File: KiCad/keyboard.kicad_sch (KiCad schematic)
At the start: 1 part

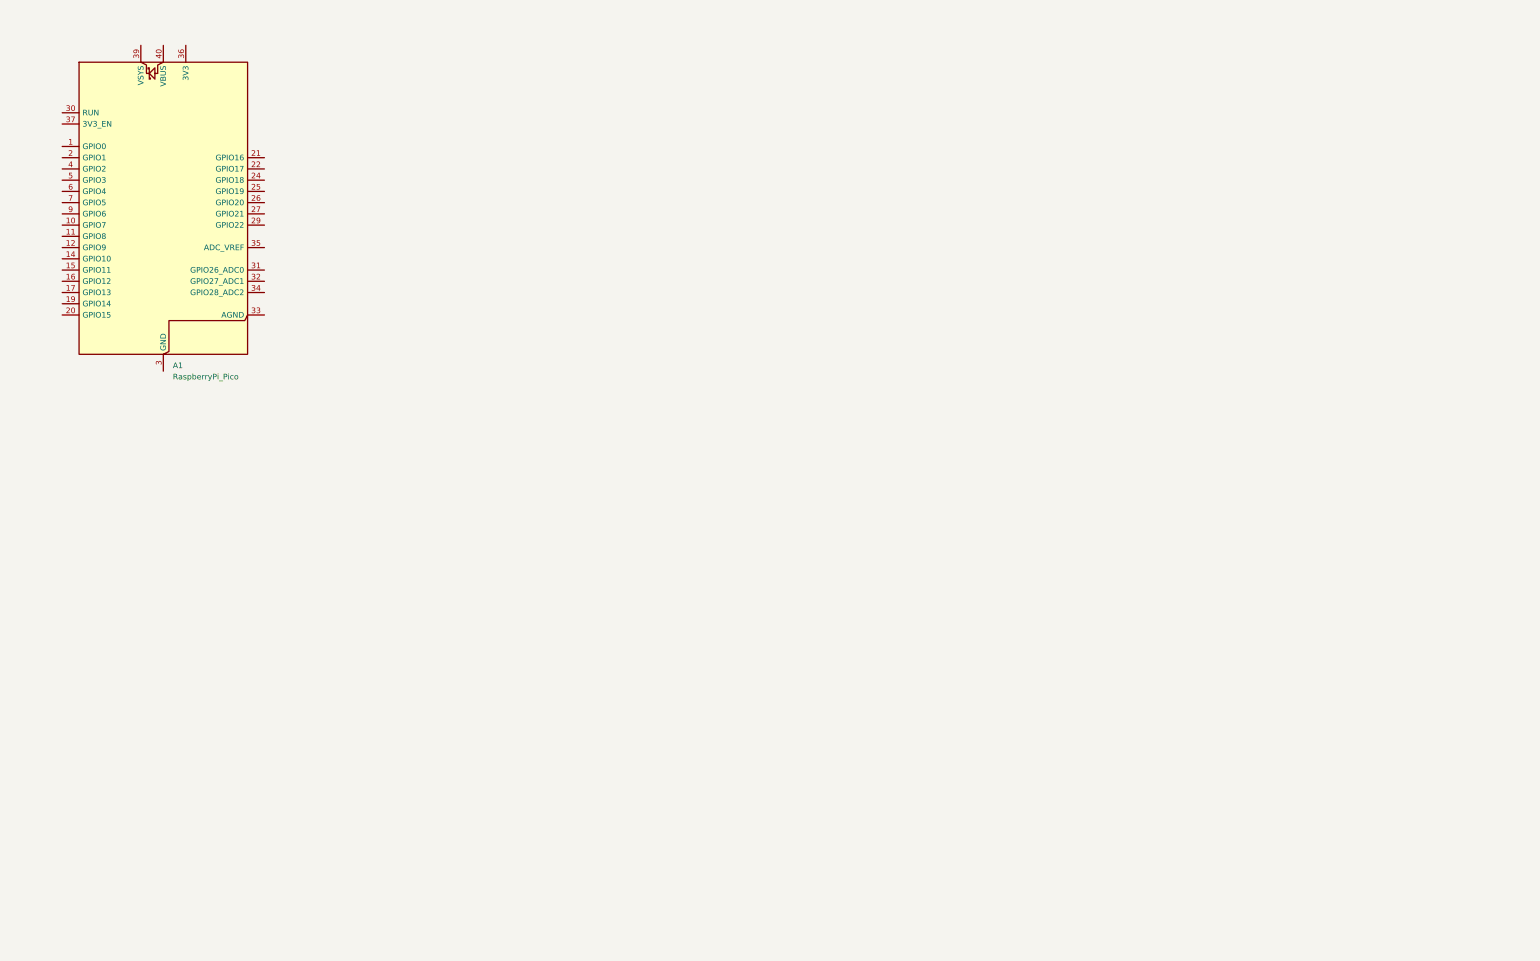
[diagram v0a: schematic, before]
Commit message: schematic
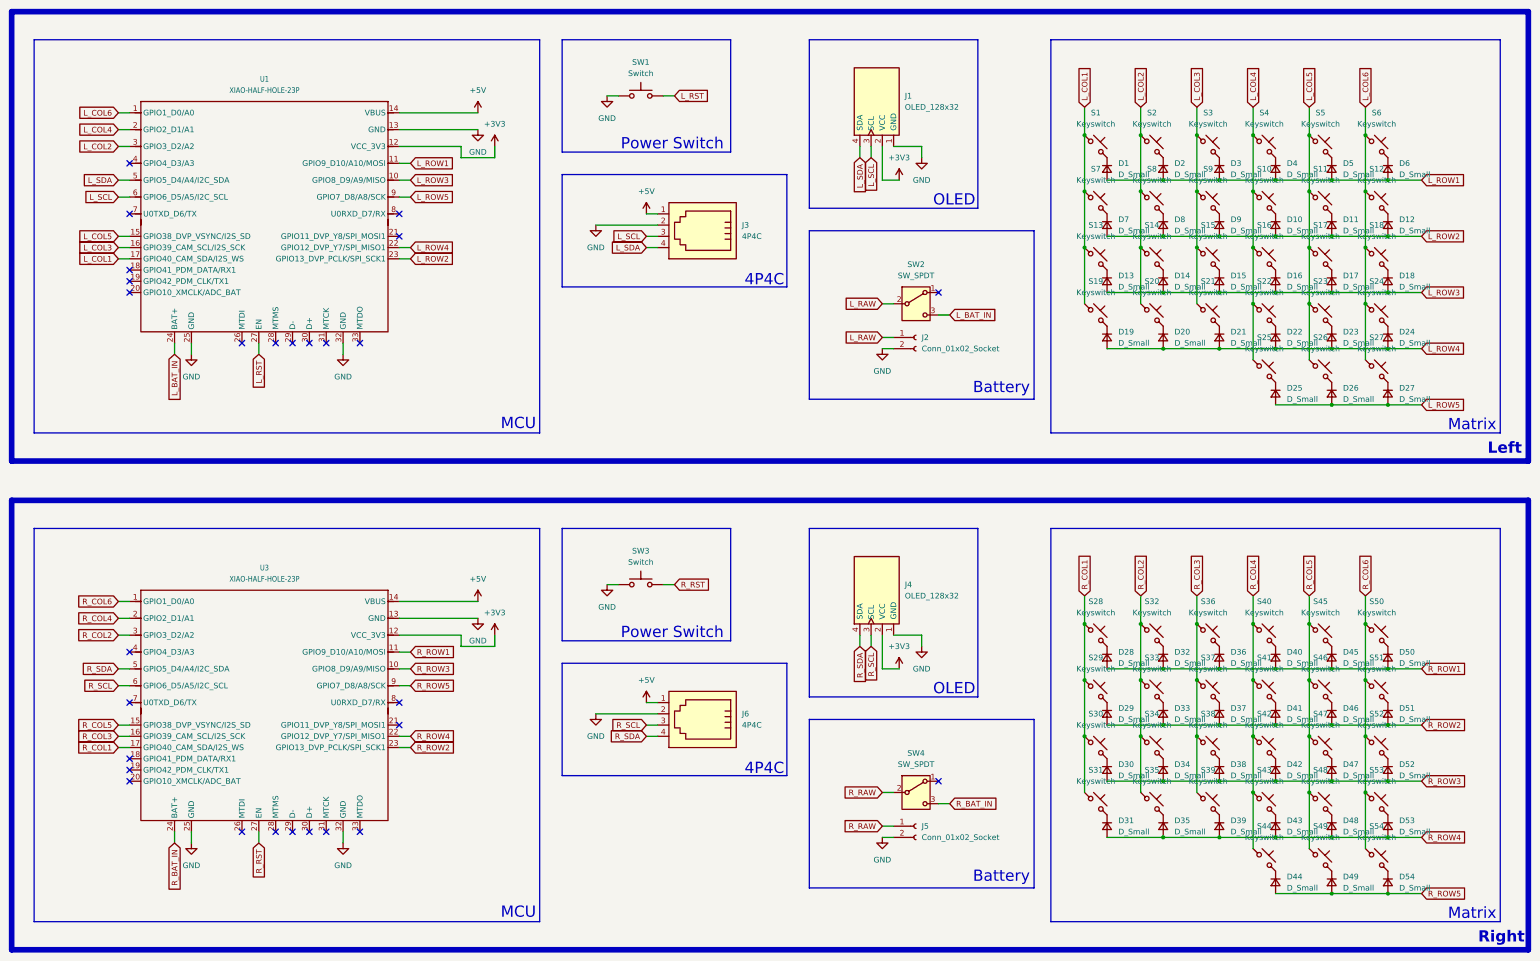
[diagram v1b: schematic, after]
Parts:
- removed A1: RaspberryPi_Pico, Module:RaspberryPi_Pico_Common_SMD, symbol MCU_Module:RaspberryPi_Pico
- added D1, D10, D11, D12, D13, D14, D15, D16, D17, D18, D19, D2, D20, D21, D22, D23, D24, D25, D26, D27, D28, D29, D3, D30, D31, D32, D33, D34, D35, D36, D37, D38, D39, D4, D40, D41, D42, D43, D44, D45, D46, D47, D48, D49, D5, D50, D51, D52, D53, D54, D6, D7, D8, D9: D_Small, chinh4thepro:ComboDiode, symbol Device:D_Small
- added J1, J4: OLED_128x32, ScottoKeebs_Components:OLED_128x32, symbol ScottoKeebs:OLED_128x32
- added J2, J5: Conn_01x02_Socket, Connector_JST:JST_PH_S2B-PH-K_1x02_P2.00mm_Horizontal, symbol Connector:Conn_01x02_Socket
- added J3, J6: 4P4C, Connector_RJ:RJ9_Evercom_5301-440xxx_Horizontal, symbol Connector:4P4C
- added S1, S10, S11, S12, S13, S14, S15, S16, S17, S18, S19, S2, S20, S21, S22, S23, S24, S25, S26, S27, S28, S29, S3, S30, S31, S32, S33, S34, S35, S36, S37, S38, S39, S4, S40, S41, S42, S43, S44, S45, S46, S47, S48, S49, S5, S50, S51, S52, S53, S54, S6, S7, S8, S9: Keyswitch, ScottoKeebs_Hotswap:Hotswap_MX, symbol ScottoKeebs:Placeholder_Keyswitch
- added SW1, SW3: Switch, chinh4thepro:reset_switch_smd_side, symbol ScottoKeebs:Placeholder_Switch
- added SW2, SW4: SW_SPDT, chinh4thepro:power_switch_smd_side, symbol Switch:SW_SPDT
- added U1, U3: XIAO-HALF-HOLE-23P, xiao ESP32S3 Plus_PCB:Xiao_ESP32S3_Plus.kicad_sym, symbol MOUDLE-SEEEDUINO-XIAO-ESP32S3-Plus:Module/XIAO-HALF-HOLE-23P
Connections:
- new net: D41.1 (K), S41.2
- new net: D28.1 (K), S28.2
- new net: D24.1 (K), S24.2
- new net: D8.1 (K), S8.2
- new net: D37.1 (K), S37.2
- new net: D52.1 (K), S52.2
- new net: D10.1 (K), S10.2
- new net: D2.1 (K), S2.2
- new net: D47.1 (K), S47.2
- new net: D29.1 (K), S29.2
- new net: D21.1 (K), S21.2
- new net: D34.1 (K), S34.2
- new net: D4.1 (K), S4.2
- new net: D20.1 (K), S20.2
- new net: D38.1 (K), S38.2
- new net: D11.1 (K), S11.2
- new net: D26.1 (K), S26.2
- new net: D49.1 (K), S49.2
- new net: D45.1 (K), S45.2
- new net: D46.1 (K), S46.2
- new net: D35.1 (K), S35.2
- new net: D12.1 (K), S12.2
- new net: D50.1 (K), S50.2
- new net: D44.1 (K), S44.2
- new net: D17.1 (K), S17.2
- new net: D13.1 (K), S13.2
- new net: D18.1 (K), S18.2
- new net: D15.1 (K), S15.2
- new net: D40.1 (K), S40.2
- new net: D23.1 (K), S23.2
- new net: D22.1 (K), S22.2
- new net: D39.1 (K), S39.2
- new net: D32.1 (K), S32.2
- new net: D27.1 (K), S27.2
- new net: D48.1 (K), S48.2
- new net: D25.1 (K), S25.2
- new net: D33.1 (K), S33.2
- new net: D5.1 (K), S5.2
- new net: D54.1 (K), S54.2
- new net: D14.1 (K), S14.2
- new net: D53.1 (K), S53.2
- new net: D16.1 (K), S16.2
- new net: D30.1 (K), S30.2
- new net: D43.1 (K), S43.2
- new net: D1.1 (K), S1.2
- new net: D6.1 (K), S6.2
- new net: D7.1 (K), S7.2
- new net: D19.1 (K), S19.2
- new net: D9.1 (K), S9.2
- new net: D36.1 (K), S36.2
- new net: D3.1 (K), S3.2
- new net: D31.1 (K), S31.2
- new net: D42.1 (K), S42.2
- new net: D51.1 (K), S51.2
- new net +3V3: J1.2 (VCC), J4.2 (VCC), U1.12 (VCC_3V3), U3.12 (VCC_3V3)
- new net +5V: J3.1, J6.1, U1.14 (VBUS), U3.14 (VBUS)
- new net GND: J1.1 (GND), J2.2 (Pin_2), J3.2, J4.1 (GND), J5.2 (Pin_2), J6.2, SW1.1, SW3.1, U1.13 (GND), U1.25 (GND), U1.32 (GND), U3.13 (GND), U3.25 (GND), U3.32 (GND)
- new net L_BAT_IN: SW2.3 (C), U1.24 (BAT+)
- new net L_COL1: S1.1, S13.1, S19.1, S7.1, U1.17 (GPIO40_CAM_SDA/I2S_WS)
- new net L_COL2: S14.1, S2.1, S20.1, S8.1, U1.3 (GPIO3_D2/A2)
- new net L_COL3: S15.1, S21.1, S3.1, S9.1, U1.16 (GPIO39_CAM_SCL/I2S_SCK)
- new net L_COL4: S10.1, S16.1, S22.1, S25.1, S4.1, U1.2 (GPIO2_D1/A1)
- new net L_COL5: S11.1, S17.1, S23.1, S26.1, S5.1, U1.15 (GPIO38_DVP_VSYNC/I2S_SD)
- new net L_COL6: S12.1, S18.1, S24.1, S27.1, S6.1, U1.1 (GPIO1_D0/A0)
- new net L_RAW: J2.1 (Pin_1), SW2.2 (B)
- new net L_ROW1: D1.2 (A), D2.2 (A), D3.2 (A), D4.2 (A), D5.2 (A), D6.2 (A), U1.11 (GPIO9_D10/A10/MOSI)
- new net L_ROW2: D10.2 (A), D11.2 (A), D12.2 (A), D7.2 (A), D8.2 (A), D9.2 (A), U1.23 (GPIO13_DVP_PCLK/SPI_SCK1)
- new net L_ROW3: D13.2 (A), D14.2 (A), D15.2 (A), D16.2 (A), D17.2 (A), D18.2 (A), U1.10 (GPIO8_D9/A9/MISO)
- new net L_ROW4: D19.2 (A), D20.2 (A), D21.2 (A), D22.2 (A), D23.2 (A), D24.2 (A), U1.22 (GPIO12_DVP_Y7/SPI_MISO1)
- new net L_ROW5: D25.2 (A), D26.2 (A), D27.2 (A), U1.9 (GPIO7_D8/A8/SCK)
- new net L_RST: SW1.2, U1.27 (EN)
- new net L_SCL: J1.3 (SCL), J3.3, U1.6 (GPIO6_D5/A5/I2C_SCL)
- new net L_SDA: J1.4 (SDA), J3.4, U1.5 (GPIO5_D4/A4/I2C_SDA)
- new net R_BAT_IN: SW4.3 (C), U3.24 (BAT+)
- new net R_COL1: S28.1, S29.1, S30.1, S31.1, U3.17 (GPIO40_CAM_SDA/I2S_WS)
- new net R_COL2: S32.1, S33.1, S34.1, S35.1, U3.3 (GPIO3_D2/A2)
- new net R_COL3: S36.1, S37.1, S38.1, S39.1, U3.16 (GPIO39_CAM_SCL/I2S_SCK)
- new net R_COL4: S40.1, S41.1, S42.1, S43.1, S44.1, U3.2 (GPIO2_D1/A1)
- new net R_COL5: S45.1, S46.1, S47.1, S48.1, S49.1, U3.15 (GPIO38_DVP_VSYNC/I2S_SD)
- new net R_COL6: S50.1, S51.1, S52.1, S53.1, S54.1, U3.1 (GPIO1_D0/A0)
- new net R_RAW: J5.1 (Pin_1), SW4.2 (B)
- new net R_ROW1: D28.2 (A), D32.2 (A), D36.2 (A), D40.2 (A), D45.2 (A), D50.2 (A), U3.11 (GPIO9_D10/A10/MOSI)
- new net R_ROW2: D29.2 (A), D33.2 (A), D37.2 (A), D41.2 (A), D46.2 (A), D51.2 (A), U3.23 (GPIO13_DVP_PCLK/SPI_SCK1)
- new net R_ROW3: D30.2 (A), D34.2 (A), D38.2 (A), D42.2 (A), D47.2 (A), D52.2 (A), U3.10 (GPIO8_D9/A9/MISO)
- new net R_ROW4: D31.2 (A), D35.2 (A), D39.2 (A), D43.2 (A), D48.2 (A), D53.2 (A), U3.22 (GPIO12_DVP_Y7/SPI_MISO1)
- new net R_ROW5: D44.2 (A), D49.2 (A), D54.2 (A), U3.9 (GPIO7_D8/A8/SCK)
- new net R_RST: SW3.2, U3.27 (EN)
- new net R_SCL: J4.3 (SCL), J6.3, U3.6 (GPIO6_D5/A5/I2C_SCL)
- new net R_SDA: J4.4 (SDA), J6.4, U3.5 (GPIO5_D4/A4/I2C_SDA)
- no-connect marks 0 -> 28
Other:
- note added: "4P4C"
- note added: "Battery"
- note added: "Left"
- note added: "MCU"
- note added: "Matrix"
- note added: "OLED"
- note added: "Power Switch"
- note added: "Right"
